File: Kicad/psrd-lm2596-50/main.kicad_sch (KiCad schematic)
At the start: 57 parts, among them K1 MAIN AC, K2 PSR1, K3 PSR2, U1 LM2596-50, U2 LM2596-50

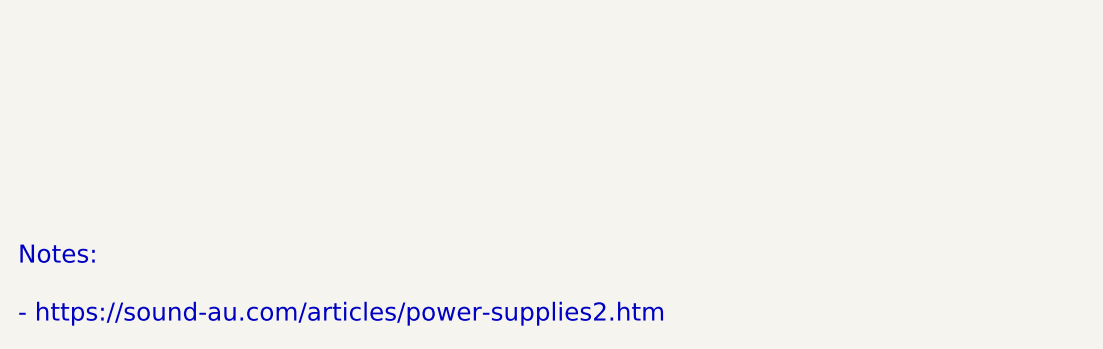
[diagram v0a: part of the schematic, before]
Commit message: Up
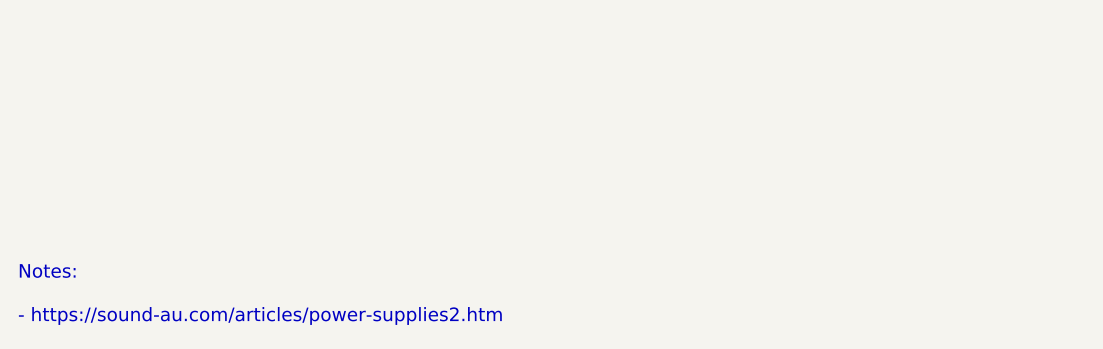
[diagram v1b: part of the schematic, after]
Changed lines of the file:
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@@
 		(effects
 			(font
-				(size 2 2)
+				(size 1.5 1.5)
 			)
 			(justify left bottom)
